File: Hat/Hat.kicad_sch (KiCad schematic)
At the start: 86 parts, among them J1 Conn_01x01_Pin, J2 Conn_01x12_Pin, J3 Conn_01x12_Pin, J4 Conn_01x06_Pin, Q1 BC547, Q10 BC547, Q3 BC547, Q4 BC547, Q6 BC547, Q7 BC547, Q8 BC547, Q8 BC557, SW1 SW_Push, SW2 SW_SPDT, U1 TL074, U13 Aux_flush, U5 4066

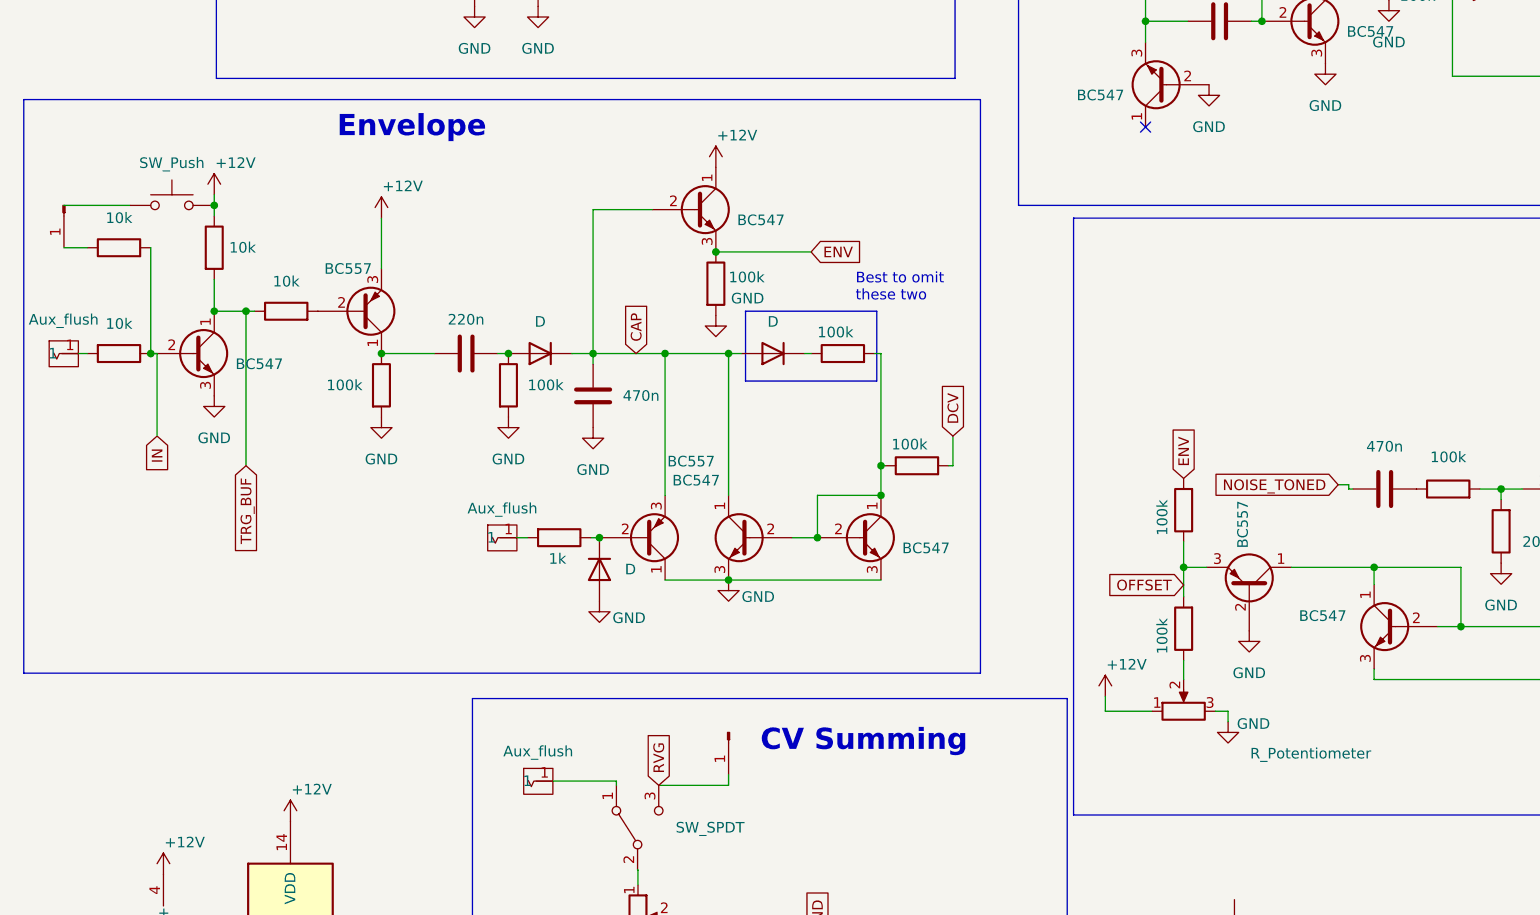
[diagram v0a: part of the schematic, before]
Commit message: Add files via upload
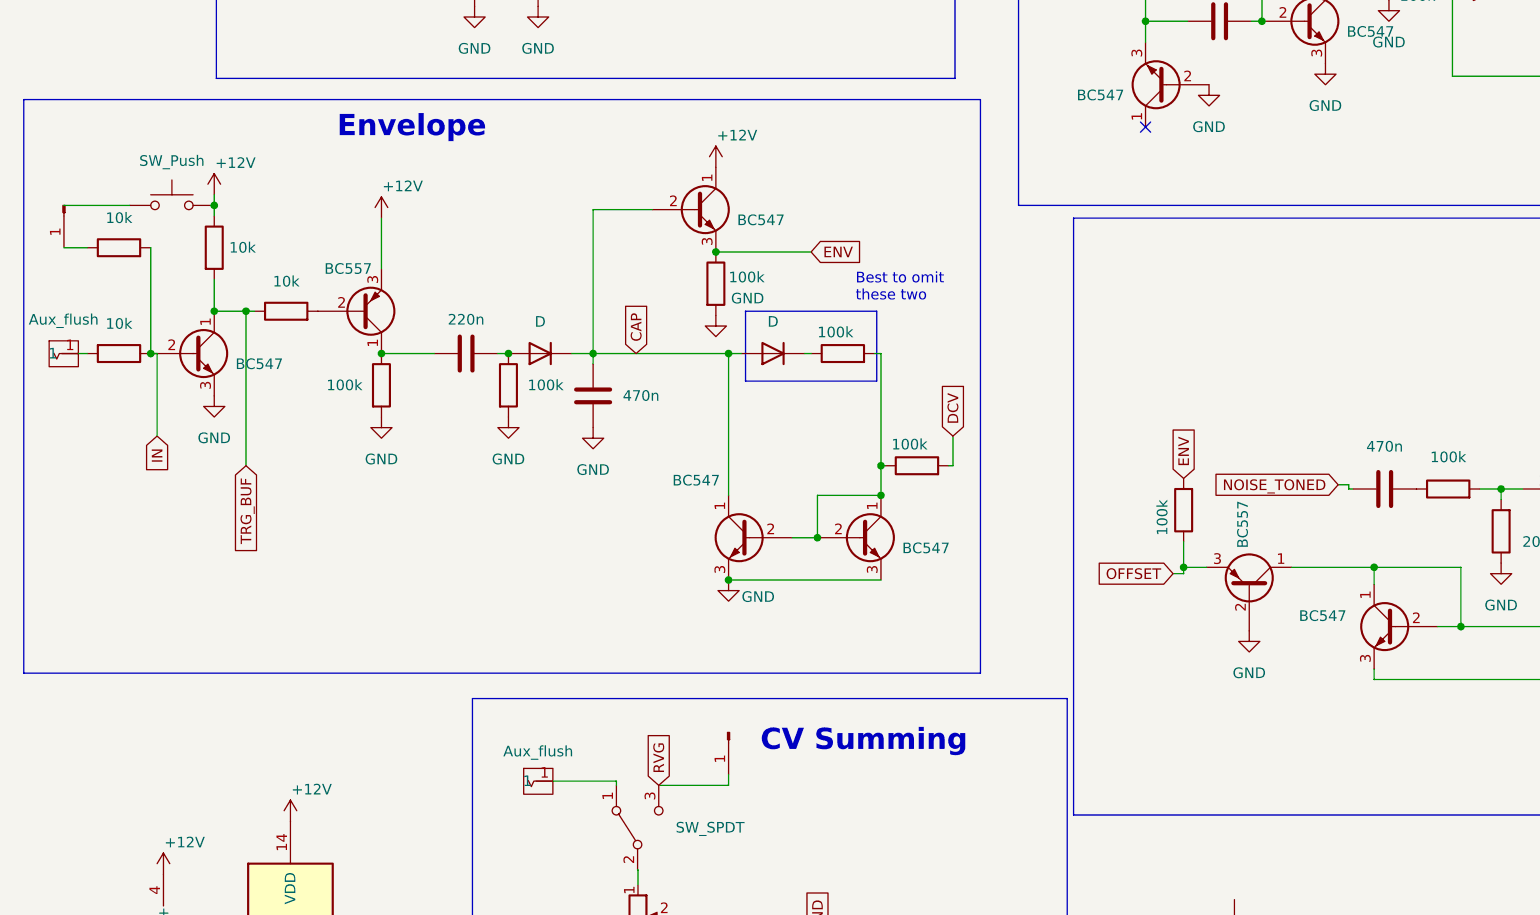
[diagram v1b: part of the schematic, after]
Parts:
- removed D8: D, Diode_THT:D_A-405_P5.08mm_Vertical_AnodeUp, symbol Device:D
- removed Q8: BC557, Package_TO_SOT_THT:TO-92_Inline_Wide, symbol Transistor_BJT:BC557
- removed R3: 100k, Resistor_THT:R_Axial_DIN0204_L3.6mm_D1.6mm_P7.62mm_Horizontal, symbol Device:R
- removed R42: 1k, Resistor_THT:R_Axial_DIN0204_L3.6mm_D1.6mm_P7.62mm_Horizontal, symbol Device:R
- removed RV4: R_Potentiometer, Library:AlpsPot, symbol Device:R_Potentiometer
- removed U13: Aux_flush, Library:3mm5 Mono Aux, symbol HEJ:Aux_flush
- SW1: footprint Library:Push_Flush -> Library:PushButton
- SW2: footprint Library:SPDT Mini -> Library:Switch
- renumbered C3 to C1, C3 to C10, C3 to C11, C3 to C2, C1 to C3, C2 to C4, C3 to C5, C3 to C6, C3 to C7, C3 to C8, C3 to C9, D8 to D1, D8 to D2, D8 to D3, D8 to D5, J1 to J5, Q3 to Q1, Q6 to Q11, Q8 to Q12, Q3 to Q13, Q3 to Q14, Q8 to Q15, Q4 to Q2, Q7 to Q3, Q8 to Q4, Q1 to Q6, Q3 to Q7, Q6 to Q8, Q8 to Q9, R3 to R1, R42 to R10, R42 to R11, R42 to R12, R2 to R13, R4 to R14, R5 to R15, R6 to R16, R6 to R17, R6 to R18, R18 to R19, R5 to R2, R22 to R21, R24 to R22, R26 to R23, R28 to R24, R3 to R25, R6 to R27, R6 to R28, R6 to R29, R38 to R3, R42 to R30, R42 to R31, R28 to R32, R6 to R33, R26 to R34, R2 to R35, R6 to R36, R39 to R4, R40 to R5, R41 to R6, R42 to R7, R3 to R8, U13 to U2, U13 to U4, U13 to U6, U13 to U7
